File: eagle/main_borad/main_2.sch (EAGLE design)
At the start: 34 parts, among them Q2 BSS123, Q3 BSS123, Q5 BSS123, Q6 BSS123, U1 XMEGA-A4TQFP

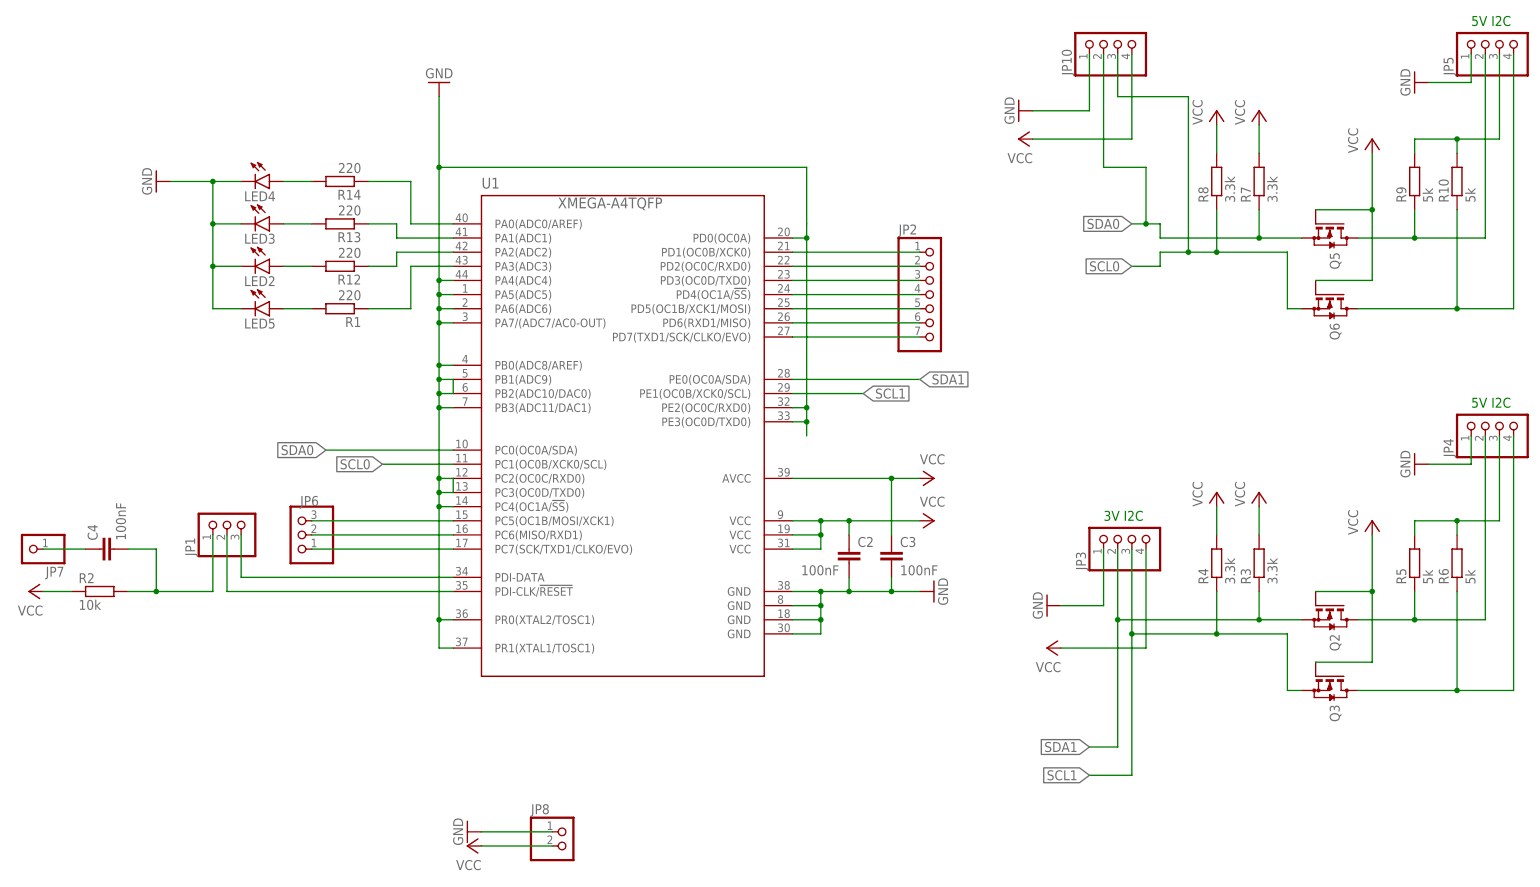
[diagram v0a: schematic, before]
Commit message: PCB layout 6.0
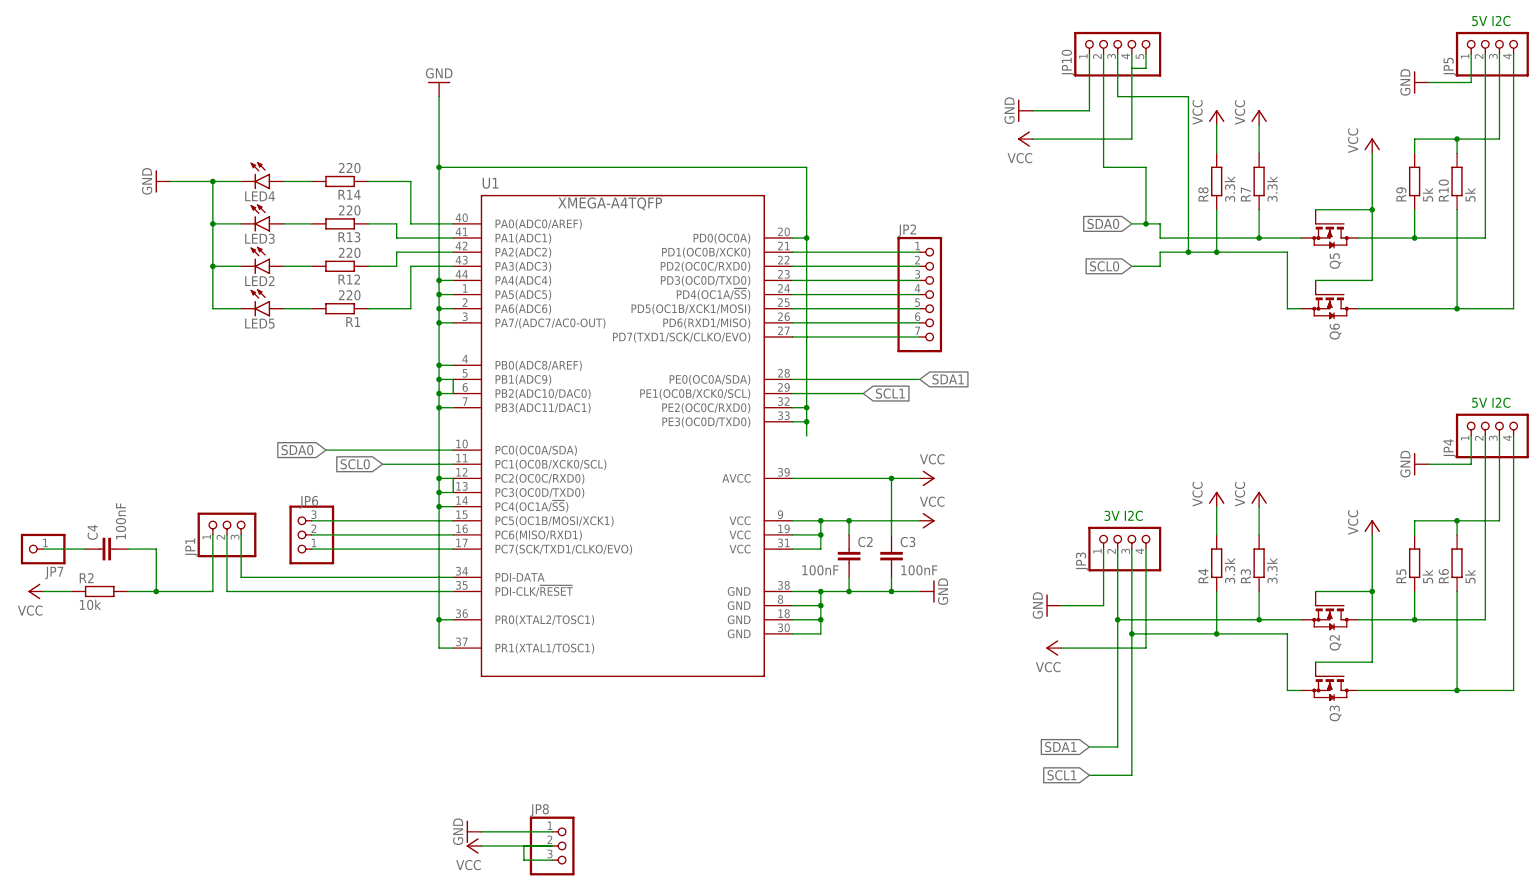
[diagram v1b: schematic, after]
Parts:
- JP10: device pinhead:PINHD-1X4 -> pinhead:PINHD-1X5
- JP8: device pinhead:PINHD-1X2 -> pinhead:PINHD-1X3
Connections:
- net VCC: now also JP10.5, JP8.3
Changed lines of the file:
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@@
 <part name="JP7" library="pinhead" deviceset="PINHD-1X1" device=""/>
 <part name="GND6" library="supply1" deviceset="GND" device=""/>
-<part name="JP8" library="pinhead" deviceset="PINHD-1X2" device=""/>
+<part name="JP8" library="pinhead" deviceset="PINHD-1X3" device=""/>
 <part name="P+1" library="supply1" deviceset="VCC" device=""/>
 <part name="GND7" library="supply1" deviceset="GND" device=""/>
-<part name="JP10" library="pinhead" deviceset="PINHD-1X4" device=""/>
+<part name="JP10" library="pinhead" deviceset="PINHD-1X5" device=""/>
 <part name="GND9" library="supply1" deviceset="GND" device=""/>
 <part name="P+13" library="supply1" deviceset="VCC" device=""/>
@@
 <instance part="JP7" gate="G$1" x="-27.94" y="35.56" rot="R180"/>
 <instance part="GND6" gate="1" x="45.72" y="119.38" rot="R180"/>
-<instance part="JP8" gate="G$1" x="68.58" y="-17.78"/>
+<instance part="JP8" gate="A" x="68.58" y="-17.78"/>
 <instance part="P+1" gate="VCC" x="50.8" y="-17.78" rot="R90"/>
 <instance part="GND7" gate="1" x="50.8" y="-15.24" rot="R270"/>
@@
 </segment>
 <segment>
-<pinref part="JP8" gate="G$1" pin="2"/>
+<pinref part="JP8" gate="A" pin="2"/>
 <wire x1="66.04" y1="-17.78" x2="53.34" y2="-17.78" width="0.1524" layer="91"/>
 <pinref part="P+1" gate="VCC" pin="VCC"/>
+<wire x1="66.04" y1="-17.78" x2="60.96" y2="-17.78" width="0.1524" layer="91"/>
+<wire x1="60.96" y1="-17.78" x2="60.96" y2="-20.32" width="0.1524" layer="91"/>
+<pinref part="JP8" gate="A" pin="3"/>
+<wire x1="60.96" y1="-20.32" x2="66.04" y2="-20.32" width="0.1524" layer="91"/>
 </segment>
 <segment>
 <pinref part="JP10" gate="A" pin="4"/>
-<wire x1="170.18" y1="124.46" x2="170.18" y2="109.22" width="0.1524" layer="91"/>
+<wire x1="170.18" y1="121.92" x2="170.18" y2="109.22" width="0.1524" layer="91"/>
 <wire x1="170.18" y1="109.22" x2="152.4" y2="109.22" width="0.1524" layer="91"/>
 <pinref part="P+13" gate="VCC" pin="VCC"/>
+<wire x1="170.18" y1="124.46" x2="170.18" y2="121.92" width="0.1524" layer="91"/>
+<wire x1="170.18" y1="121.92" x2="172.72" y2="121.92" width="0.1524" layer="91"/>
+<pinref part="JP10" gate="A" pin="5"/>
+<wire x1="172.72" y1="121.92" x2="172.72" y2="124.46" width="0.1524" layer="91"/>
 </segment>
 </net>
@@
 </segment>
 <segment>
-<pinref part="JP8" gate="G$1" pin="1"/>
+<pinref part="JP8" gate="A" pin="1"/>
 <wire x1="66.04" y1="-15.24" x2="53.34" y2="-15.24" width="0.1524" layer="91"/>
 <pinref part="GND7" gate="1" pin="GND"/>
